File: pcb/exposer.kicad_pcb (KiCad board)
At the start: 2 copper layers, 10 parts, among them IC1 ULN2065B, J1 Conn_01x04_Female, J2 Conn_01x02, SW1 SW_Push, SW2 SW_Push, SW3 SW_Push, SW4 SW_SPST

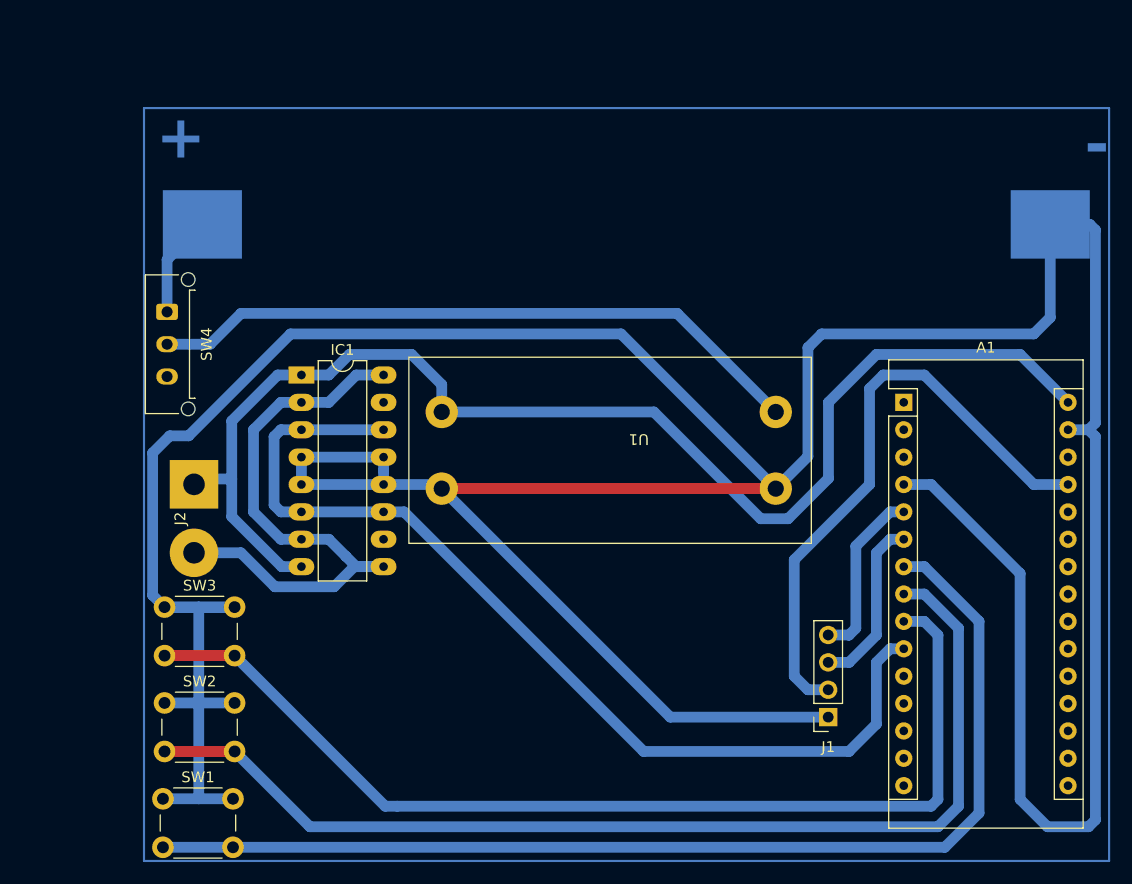
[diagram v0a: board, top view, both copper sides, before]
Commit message: encoder pcb
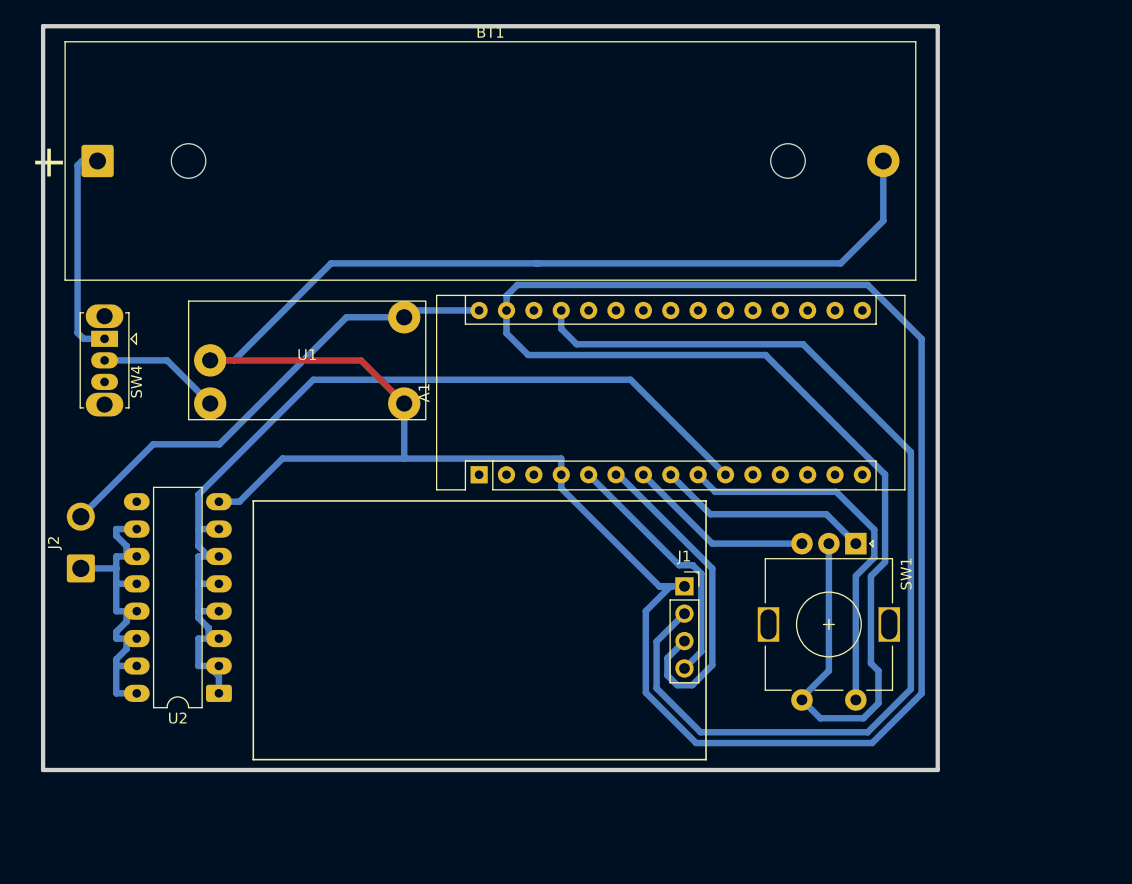
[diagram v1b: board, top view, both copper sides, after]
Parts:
- removed IC1: ULN2065B, Package_DIP:DIP-16_W7.62mm_LongPads
- removed SW2, SW3: SW_Push, Button_Switch_THT:SW_PUSH_6mm_H5mm
- added U2: ULN2003A, Package_DIP:DIP-16_W7.62mm_LongPads, F.Cu at (29.8, 75.9)
- BT1: footprint Battery:BatteryHolder_Keystone_1042_1x18650 -> Battery:BatteryHolder_MPD_BH-18650-PC; moved to F.Cu
- J2: footprint Connector_Wire:SolderWirePad_1x02_P7.62mm_Drill2mm -> Connector_Wire:SolderWire-0.75sqmm_1x02_P4.8mm_D1.25mm_OD2.3mm
- SW1: value SW_Push -> RotaryEncoder_Switch; footprint Button_Switch_THT:SW_PUSH_6mm_H5mm -> Rotary_Encoder:RotaryEncoder_Alps_EC11E-Switch_Vertical_H20mm
- SW4: footprint Connector_Molex:Molex_Micro-Fit_3.0_43650-0315_1x03_P3.00mm_Vertical -> Button_Switch_THT:SW_Slide_SPDT_Straight_CK_OS102011MS2Q
- moved SW1 68.5 mm to (88.9, 62.0), turned to -90 degrees
- moved BT1 49.4 mm to (18.6, 26.5)
- moved A1 40.0 mm to (54.0, 55.6), turned to 90 degrees
- moved U1 31.5 mm to (38.0, 45.0), turned to 0 degrees
- moved J1 18.0 mm to (73.0, 66.0), turned to 0 degrees
- moved J2 13.1 mm to (17.0, 64.3), turned to 90 degrees
- moved SW4 6.31 mm to (19.2, 43.0)
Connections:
- J2 pad 1: +12V -> Net-(J2-Pin_1)
- J2 pad 2: Net-(IC1-O1) -> +12V
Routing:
- net Net-(A1-D4): track 103.9 -> 17.4 mm
- net Net-(A1-D5): track 100.2 -> 19.8 mm
- net +12V: track 121.2 -> 44.9 mm
- net Net-(A1-D6): track 96.7 -> 34.9 mm
- net Net-(IC1-O1): track 55.6 -> 0.00 mm
- net +BATT: track 61.4 -> 11.5 mm
- net +5V: track 56.4 -> 95.8 mm
- net Net-(J2-Pin_1): track 0.00 -> 33.0 mm
- net GND: track 380.0 -> 354.5 mm
- net Net-(A1-D3): track 16.2 -> 30.7 mm
- net Net-(BT1-+): track 9.47 -> 20.3 mm
- net Net-(A1-D2): track 16.2 -> 23.7 mm
- net Net-(A1-D7): track 92.0 -> 88.0 mm
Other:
- board outline added: 83 x 69 mm
- board text removed: "+"
- board text removed: "-"
